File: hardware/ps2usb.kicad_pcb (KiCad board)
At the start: 2 copper layers, 40 x 55 mm, 21 parts, among them J1 DIN8, J2 USB1035, J3 DIN8, J4 DB9_Female_MountingHoles, U1 CH559L-less, U2 MAX232

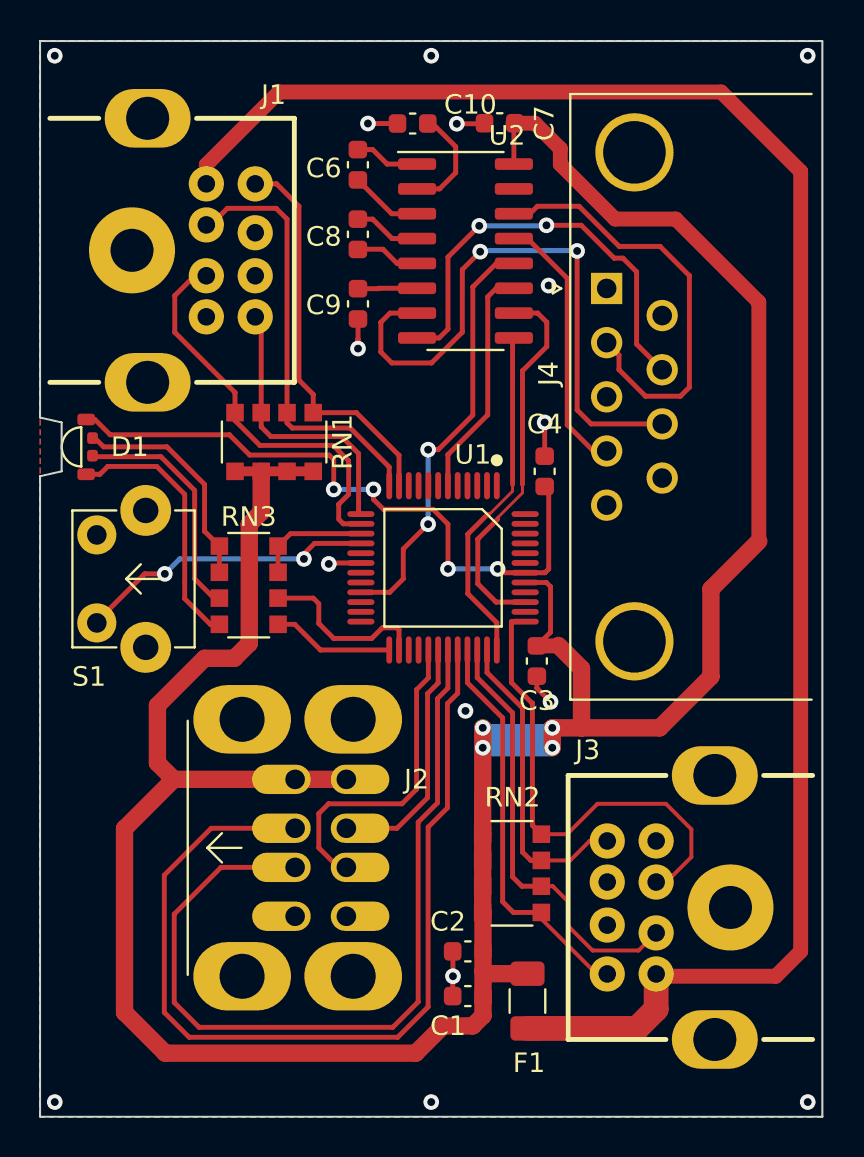
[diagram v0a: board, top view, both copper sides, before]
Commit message: Internal version, replaced connectors with headers
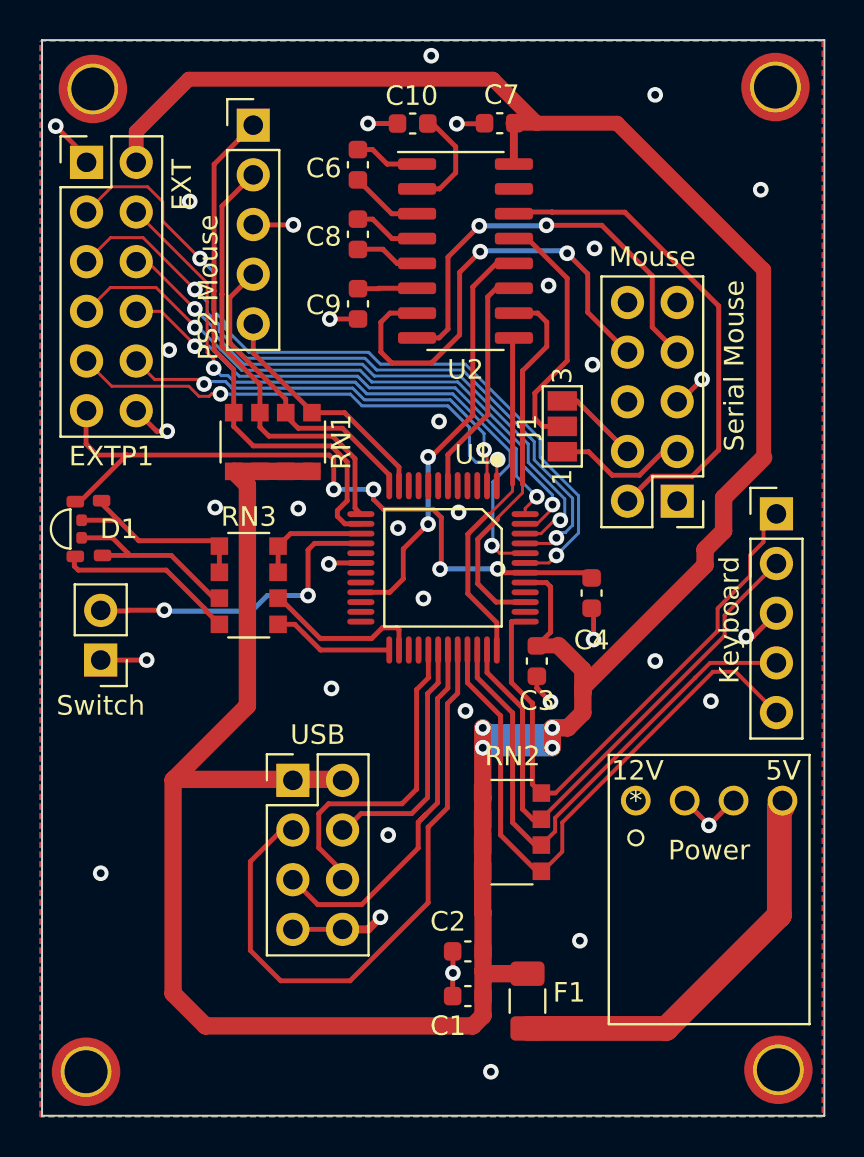
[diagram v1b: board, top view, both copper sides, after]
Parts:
- removed S1: RATACSWITCH, ps2usb:TS11
- added ?: , , F.Cu at (100.2, 93.8)
- added ?: , , F.Cu at (100.1, 91.0)
- added EXT: EXTP1, Connector_PinHeader_2.54mm:PinHeader_2x06_P2.54mm_Vertical, F.Cu at (99.4, 73.7)
- added PS2 Mouse: PS2 Mouse, Connector_PinHeader_2.54mm:PinHeader_1x05_P2.54mm_Vertical, F.Cu at (107.9, 71.8)
- added Power: CONN_171826-4_TYCO_TYC, ps2usb:171826-4, F.Cu at (127.5, 106.3)
- added REF**: MountingHole_2.2mm_M2_ISO7380_Pad_TopOnly, MountingHole:MountingHole_2.2mm_M2_ISO7380_Pad_TopOnly, F.Cu at (134.8, 120.1)
- added REF**: MountingHole_2.2mm_M2_ISO7380_Pad_TopOnly, MountingHole:MountingHole_2.2mm_M2_ISO7380_Pad_TopOnly, F.Cu at (99.3, 120.2)
- added REF**: MountingHole_2.2mm_M2_ISO7380_Pad_TopOnly, MountingHole:MountingHole_2.2mm_M2_ISO7380_Pad_TopOnly, F.Cu at (99.7, 70.0)
- added REF**: MountingHole_2.2mm_M2_ISO7380_Pad_TopOnly, MountingHole:MountingHole_2.2mm_M2_ISO7380_Pad_TopOnly, F.Cu at (134.6, 69.8)
- added Switch: PinHeader_1x02_P2.54mm_Vertical, Connector_PinHeader_2.54mm:PinHeader_1x02_P2.54mm_Vertical, F.Cu at (100.1, 99.2)
- J1: value DIN8 -> J1; footprint ps2usb:DIN8 -> Jumper:SolderJumper-3_P1.3mm_Open_Pad1.0x1.5mm_NumberLabels
- Keyboard: renamed from J3; value DIN8 -> Keyboard; footprint ps2usb:DIN8 -> Connector_PinHeader_2.54mm:PinHeader_1x05_P2.54mm_Vertical
- Serial Mouse: renamed from J4; value DB9_Female_MountingHoles -> Mouse; footprint Connector_Dsub:DSUB-9_Female_Horizontal_P2.77x2.84mm_EdgePinOffset7.70mm_Housed_MountingHolesOffset9.12mm -> Connector_PinHeader_2.54mm:PinHeader_2x05_P2.54mm_Vertical
- USB: renamed from J2; value USB1035 -> USB; footprint ps2usb:USB1035 -> Connector_PinHeader_2.54mm:PinHeader_2x04_P2.54mm_Vertical
- moved J1 28.2 mm to (123.7, 87.2)
- moved Keyboard 20.3 mm to (134.7, 91.7), turned to 0 degrees
- moved Serial Mouse 11.5 mm to (129.6, 91.0), turned to 180 degrees
- moved C4 6.67 mm to (125.2, 95.7), turned to 90 degrees
- moved USB 6.36 mm to (109.9, 105.3), turned to 0 degrees
- moved D1 4.24 mm to (98.8, 92.5)
- moved RN2 2.10 mm to (121.1, 108.0)
- moved RN1 0.07 mm to (108.9, 88.0)
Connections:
- J1 pad 1: /DIN1-1 -> unconnected-(J4-Pad3)
- J1 pad 2: /DIN1-2 -> /DTR_232
- J1 pad 3: GND -> /DTR_232
- Keyboard pad 2: /DIN2-2 -> /DIN2-6
- Keyboard pad 4: unconnected-(J3-Pad4) -> /DIN2-2
- Keyboard pad 5: Net-(F1-Pad2) -> /DIN2-8
- U1 pad 1: (no net) -> /EXT7
- U1 pad 2: (no net) -> /EXT8
- U1 pad 43: (no net) -> /EXT1
- U1 pad 44: (no net) -> /EXT2
- U1 pad 45: (no net) -> /EXT3
- U1 pad 46: (no net) -> /EXT4
- U1 pad 47: (no net) -> /EXT5
- U1 pad 48: (no net) -> /EXT6
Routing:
- net Net-(F1-Pad2): track 91.2 -> 21.0 mm
- net /EXT1: track 0.00 -> 40.6 mm, vias 0 -> 2
- net /EXT3: track 0.00 -> 36.4 mm, vias 0 -> 2
- net /EXT2: track 0.00 -> 34.8 mm, vias 0 -> 2
- net /EXT5: track 0.00 -> 31.7 mm, vias 0 -> 2
- net /EXT4: track 0.00 -> 31.2 mm, vias 0 -> 2
- net /EXT6: track 0.00 -> 26.4 mm, vias 0 -> 2
- net /EXT7: track 0.00 -> 25.5 mm, vias 0 -> 2
- net Net-(J2-Pad3B): track 43.9 -> 19.3 mm
- net /EXT8: track 0.00 -> 22.2 mm, vias 0 -> 2
- net GND: track 13.6 -> 33.0 mm, vias 15 -> 37
- net Net-(J2-Pad2B): track 48.2 -> 32.3 mm
- net +5V: track 149.2 -> 162.8 mm
- net /DIN2-6: track 16.0 -> 28.1 mm
- net /DIN2-8: track 20.7 -> 31.7 mm
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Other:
- outline, holes or cut-outs redrawn
